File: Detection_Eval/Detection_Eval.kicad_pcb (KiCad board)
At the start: 2 copper layers, 55 x 55 mm, 52 parts, among them J1 USB4085-GF-A_REVB, Q2 PMOS, U1 SN74LVC1G08DCKR, U6 ESP8266, U7 TPS61022

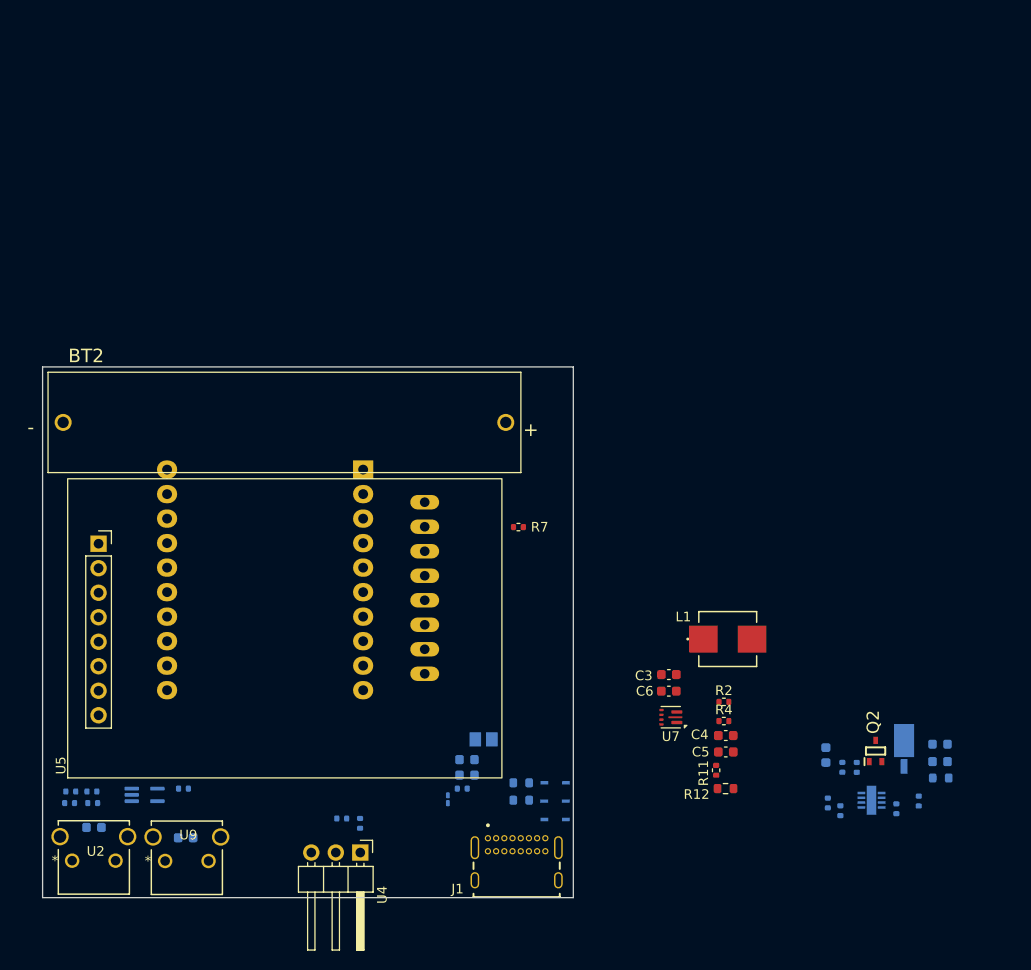
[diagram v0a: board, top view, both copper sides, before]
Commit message: LAYOUT DONE
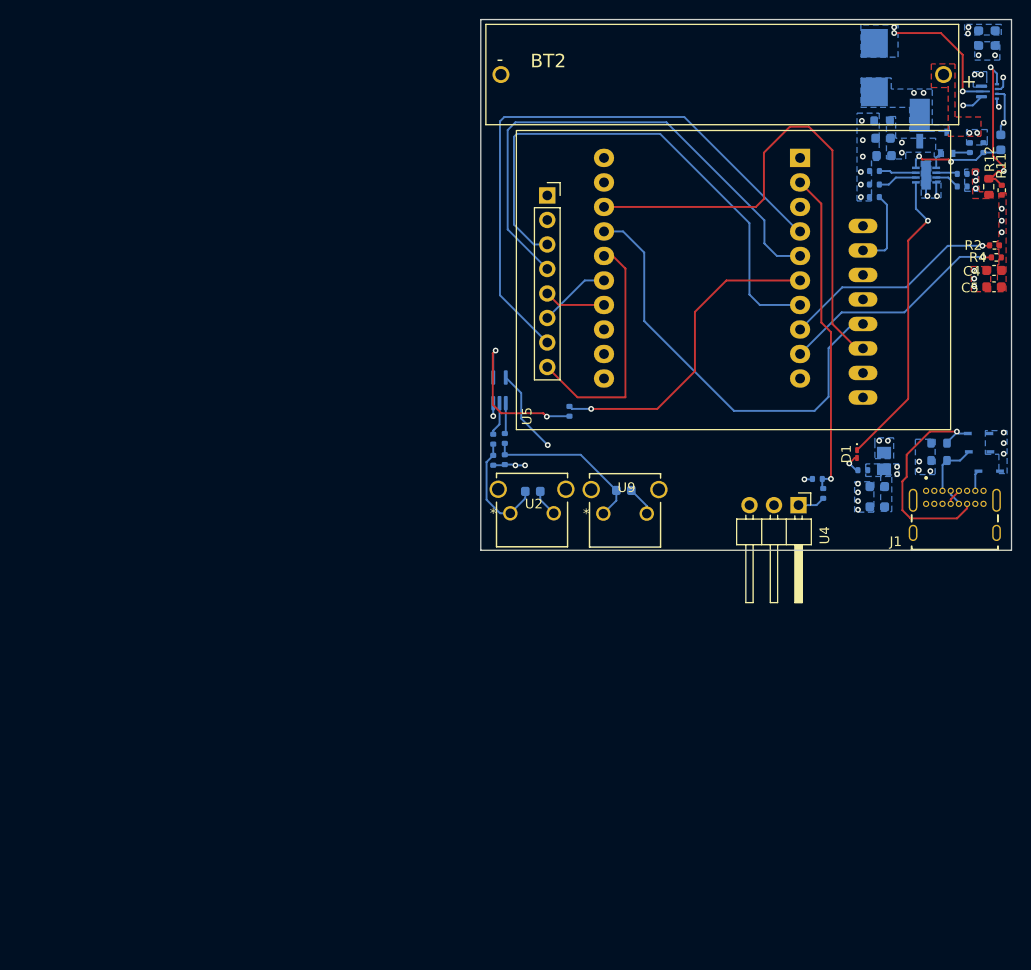
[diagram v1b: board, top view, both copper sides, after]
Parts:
- C3, C6, L1, Q2, R7, U7: moved to B.Cu
- D1: moved to F.Cu
- moved C6 74.9 mm to (141.0, 89.9), turned to 90 degrees
- moved C3 74.1 mm to (142.7, 89.9), turned to 90 degrees
- moved U7 72.7 mm to (141.9, 95.5), turned to 0 degrees
- moved R16 68.4 mm to (131.0, 98.5), turned to 180 degrees
- moved R12 68.1 mm to (142.1, 105.3), turned to -90 degrees
- moved R11 67.0 mm to (143.4, 105.7), turned to 90 degrees
- moved C9 66.0 mm to (143.3, 100.7)
- moved R18 65.9 mm to (141.5, 101.3), turned to -90 degrees
- moved R21 65.7 mm to (130.2, 103.7), turned to 0 degrees
- moved R17 65.3 mm to (140.1, 101.3), turned to 90 degrees
- moved R20 65.1 mm to (139.3, 104.0), turned to 180 degrees
- moved U8 65.0 mm to (135.6, 104.1)
- moved R22 65.0 mm to (130.2, 105.1), turned to 0 degrees
- moved C7 64.9 mm to (131.1, 100.3), turned to 180 degrees
- moved R19 64.9 mm to (139.3, 105.3), turned to 180 degrees
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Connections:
- C1 pad 1: +BATT -> +5V
- C2 pad 1: +BATT -> +5V
- C3 pad 1: +VCC -> VCC
- C6 pad 1: +VCC -> VCC
- L1 pad 1: +VCC -> VCC
- U1 pad 5: +BATT -> +5V
- U2 pad 2: +BATT -> +5V
- U7 pad 5: +VCC -> VCC
- U7 pad 7: +VCC -> VCC
- U9 pad 2: +BATT -> +5V
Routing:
- net RESET: track 0.00 -> 61.1 mm
- net HSPI_MOSI: track 0.00 -> 54.9 mm
- net HSPI_CLK: track 0.00 -> 53.9 mm
- net SCL_ACCEL: track 0.00 -> 53.2 mm
- net SDA_ACCEL: track 0.00 -> 45.4 mm
- net ECG: track 0.00 -> 34.0 mm, vias 0 -> 1
- net Net-(U6-GPIO12): track 0.00 -> 33.1 mm, vias 0 -> 1
- net Net-(D1-K): track 0.00 -> 31.3 mm, vias 0 -> 1
- net BACKLIGHT: track 0.00 -> 25.5 mm
- net Net-(U6-VBAT): track 0.00 -> 24.0 mm, vias 0 -> 1
- net Net-(U6-VIN): track 0.00 -> 23.4 mm, vias 0 -> 1
- net /Battery/CC2: track 0.00 -> 22.9 mm, vias 0 -> 1
- net Net-(C1-Pad2): track 0.00 -> 17.2 mm
- net FAILSAFE: track 0.00 -> 17.1 mm, vias 0 -> 2
- net GND: track 0.00 -> 16.7 mm, vias 0 -> 32
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- added copper zone on In2.Cu, net +3V3
- added copper zone on B.Cu, net +5V
- added copper zone on F.Cu, net +5V
- added copper zone on In2.Cu, net +5V
- added copper zone on B.Cu, net GND
- added copper zone on F.Cu, net GND
- added copper zone on In1.Cu, net GND
- added copper zone on B.Cu, net Net-(BT2-PadP)
- added copper zone on F.Cu, net Net-(BT2-PadP)
- added copper zone on B.Cu, net Net-(U7-SW)
- added copper zone on B.Cu, net VBUS
- added copper zone on B.Cu, net VCC
- added copper zone on In2.Cu, net VCC
- added copper zone on B.Cu, net VDD
- added copper zone on In2.Cu, net VDD
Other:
- copper layers 2 -> 4
